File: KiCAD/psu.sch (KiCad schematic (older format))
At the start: 26 parts

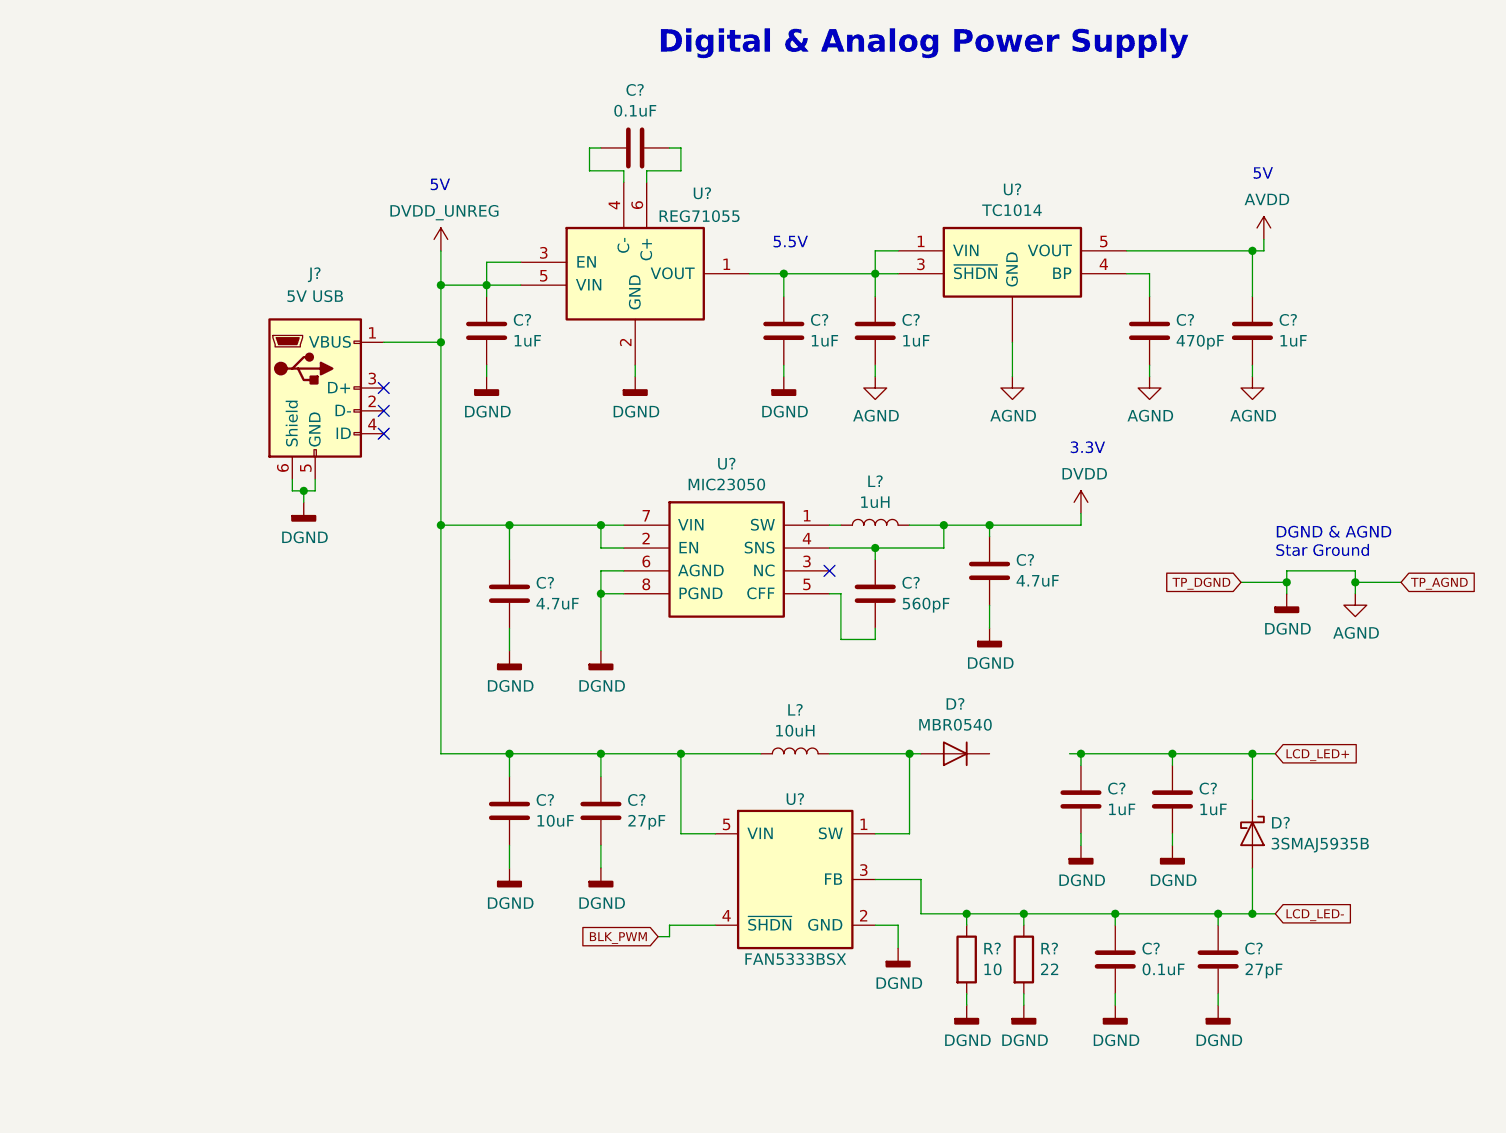
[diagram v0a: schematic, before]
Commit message: Decoupling caps & more
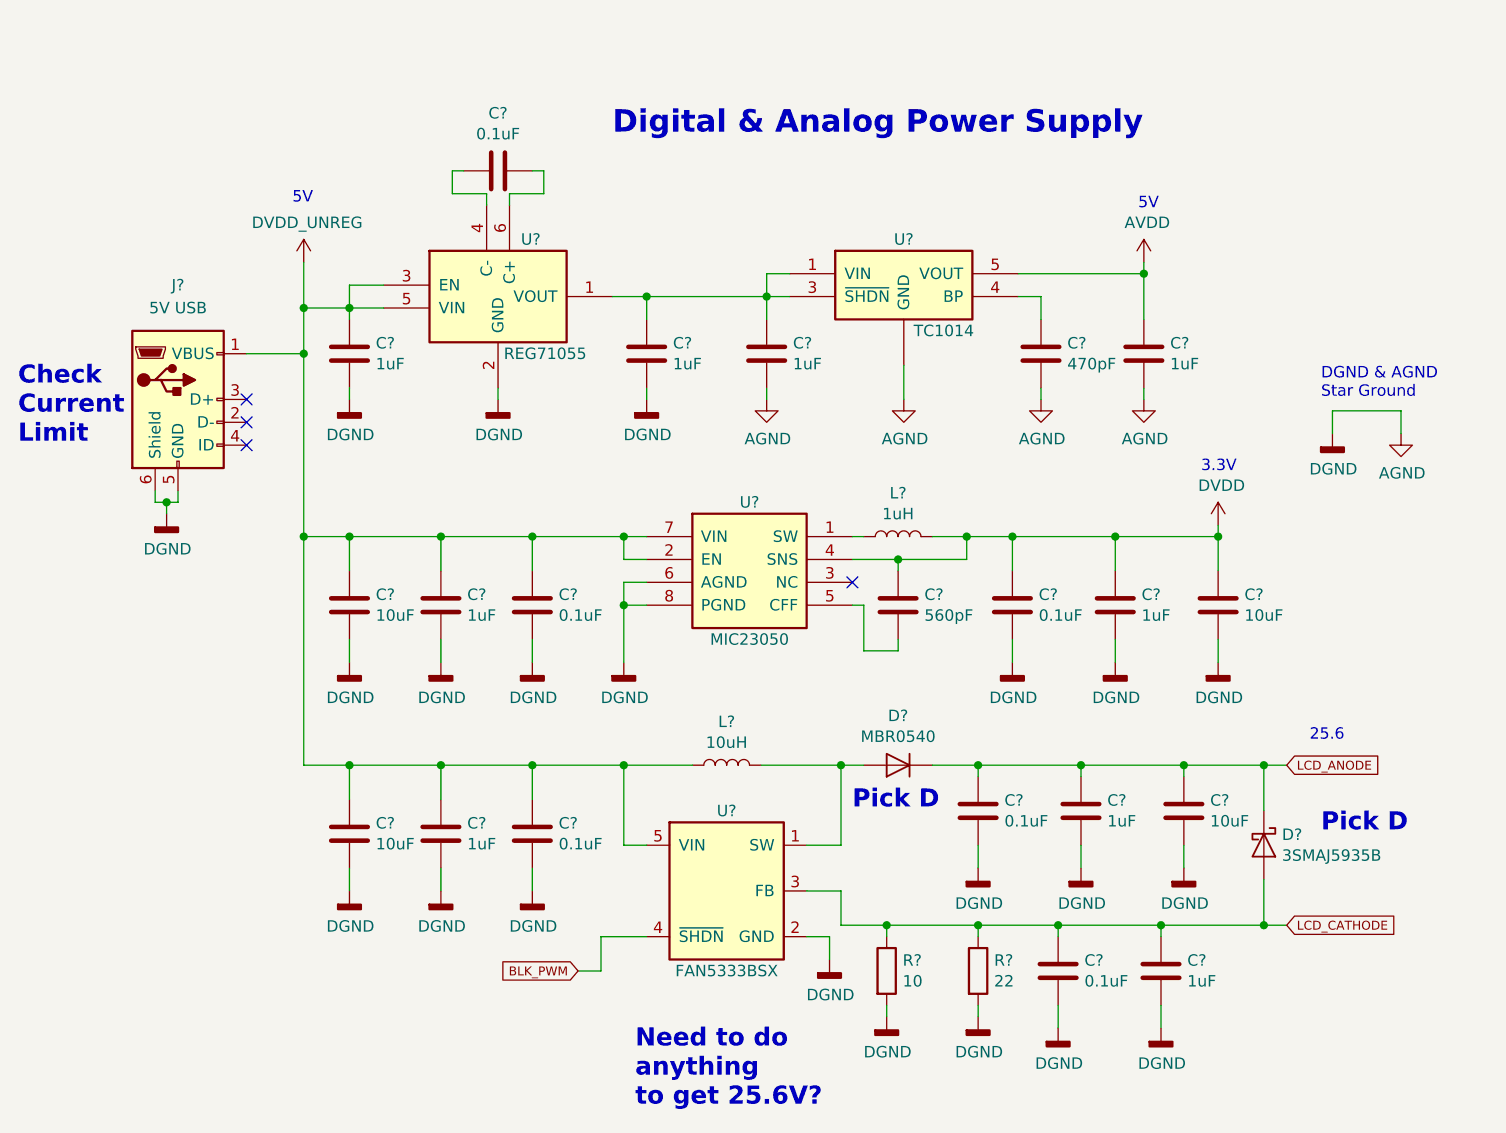
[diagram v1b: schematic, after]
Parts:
- removed C? (x2): 4.7uF, symbol Device:C
- removed C?: 10uF, symbol Device:C
- removed C? (x2): 1uF, symbol Device:C
- removed C?: 0.1uF, symbol Device:C
- removed C? (x2): 27pF, symbol Device:C
- added C? (x4): 10uF, symbol Device:C
- added C? (x5): 0.1uF, symbol Device:C
- added C? (x5): 1uF, symbol Device:C
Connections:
- net LCD_LED+ is gone; now on net LCD_ANODE: D?.1 (K)
- net AGND: now also C?.2, C?.2, C?.2, C?.2, C?.2, C?.2, C?.2, C?.2, C?.2, C?.2, C?.2, C?.2, C?.2, C?.2
- net DVDD: now also C?.1, C?.1, C?.1
- net DVDD_UNREG: now also C?.1, C?.1, C?.1, C?.1, C?.1, C?.1
- net LCD_ANODE: now reaches D?.1 (K)
- net LCD_ANODE: now also C?.1, C?.1, C?.1
- net LCD_LED- renamed LCD_CATHODE
- net LCD_CATHODE: now also C?.1, C?.1
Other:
- note added: "25.6"
- note added: "Check\nCurrent\nLimit"
- note added: "Need to do\nanything\nto get 25.6V?"
- note added: "Pick D"
- note removed: "5.5V"
- moved on the sheet: C?, D?, J?, L?, R?, U?
